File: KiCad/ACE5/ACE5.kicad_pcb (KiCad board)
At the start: 2 copper layers, 160 x 100 mm, 90 parts, among them Q1 2N3904, Q3 BC237, U1 LM7805_TO220, X1 CRYSTALHC49U-V 6.556MHz, X2 5MHz

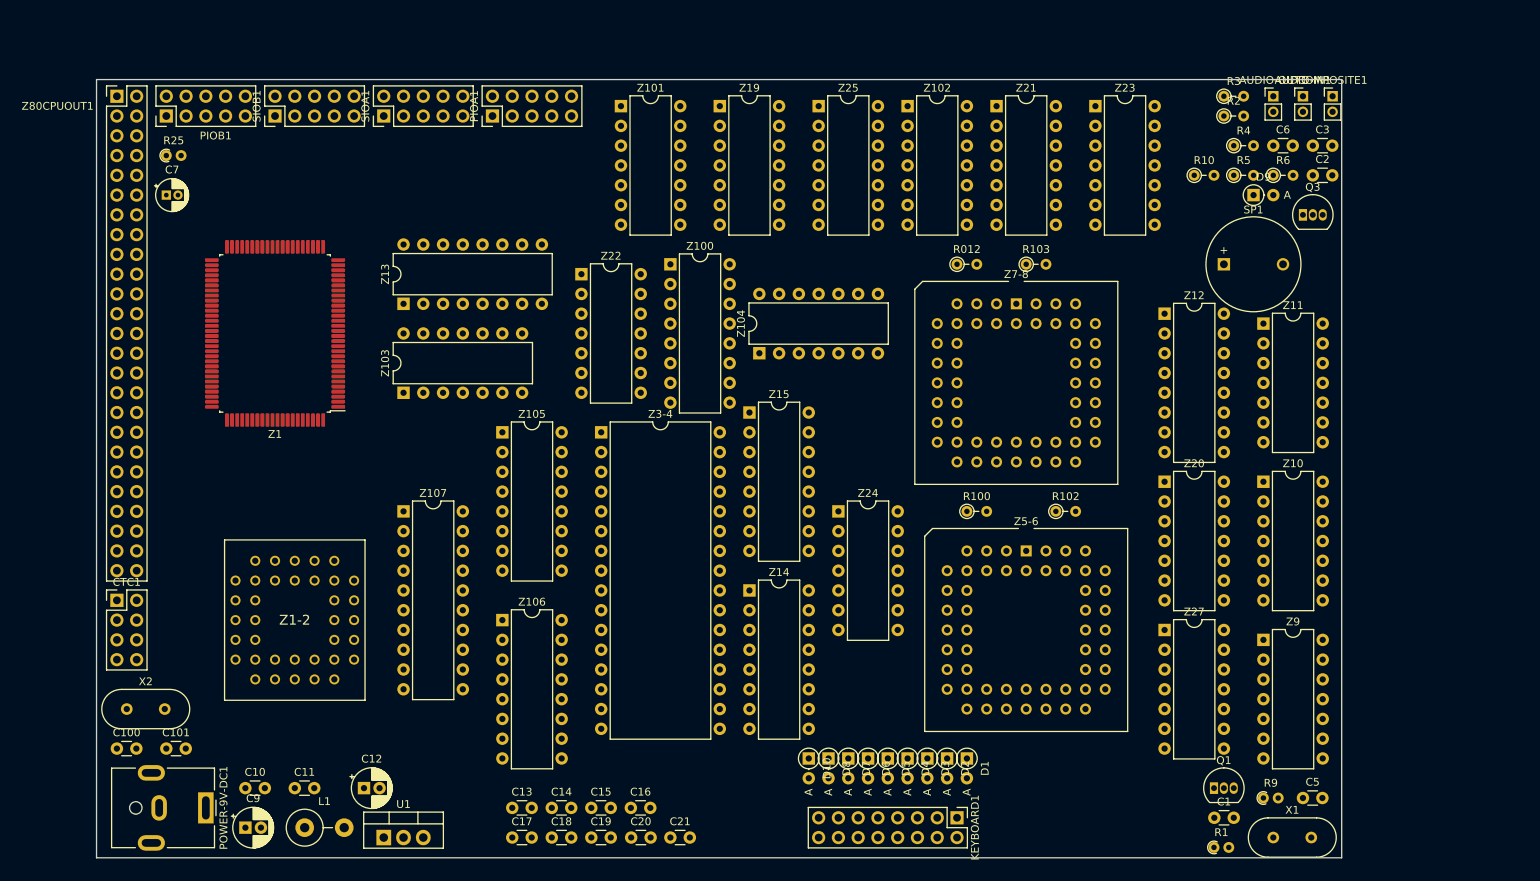
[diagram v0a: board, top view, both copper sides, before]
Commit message: UPdate to latest version.
Signed-off-by: John Bradley <flypie@rocketmail.com>
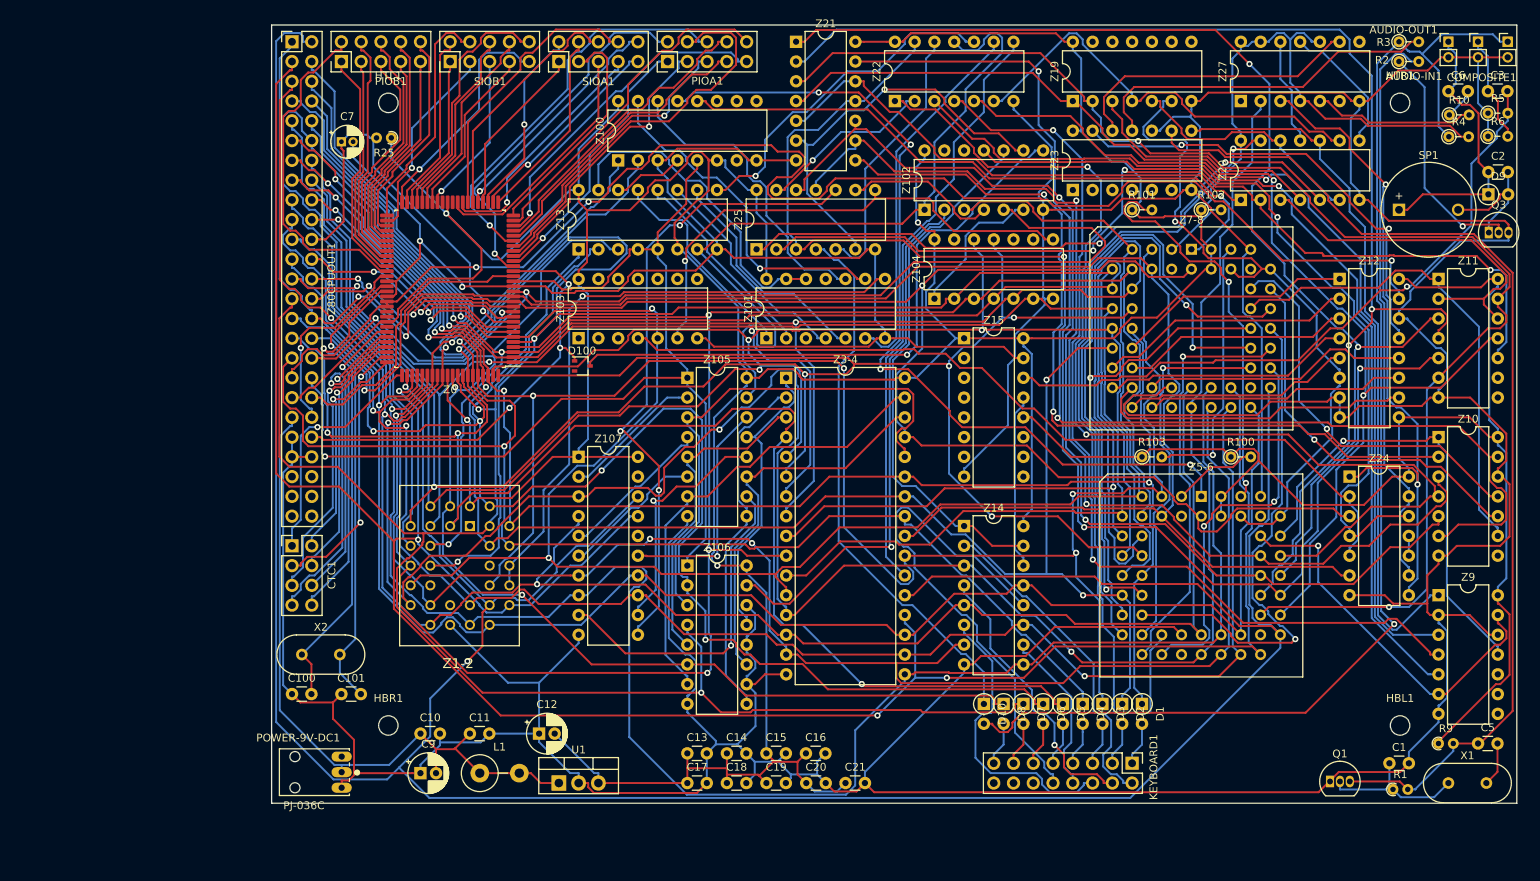
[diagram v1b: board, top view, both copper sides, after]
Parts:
- added D100: BAT54W, Package_TO_SOT_SMD:SOT-323_SC-70, F.Cu at (130.9, 91.8)
- added HBL1: MountingHole, MountingHole:MountingHole_2.5mm, F.Cu at (236.0, 138.0)
- added HBR1: MountingHole, MountingHole:MountingHole_2.5mm, F.Cu at (106.0, 138.0)
- added HTL1: MountingHole, MountingHole:MountingHole_2.5mm, F.Cu at (106.0, 58.0)
- added HTR1: MountingHole, MountingHole:MountingHole_2.5mm, F.Cu at (236.0, 58.0)
- L1: value L -> 100 nH
- POWER-9V-DC1: value Conn_01x02 -> PJ-036C; footprint Connector_BarrelJack:BarrelJack_CUI_PJ-063AH_Horizontal -> cuipj:CUI_PJ-036C
- moved Z27 68.7 mm to (215.5, 57.8), turned to 90 degrees
- moved Z24 65.8 mm to (229.5, 106.0)
- moved Z22 46.0 mm to (171.1, 57.8), turned to 90 degrees
- moved Z19 45.4 mm to (193.9, 57.8), turned to 90 degrees
- moved R101 40.0 mm to (201.6, 71.7)
- moved Z20 37.5 mm to (215.5, 70.5), turned to 90 degrees
- moved Z101 35.2 mm to (154.6, 88.2), turned to 90 degrees
- moved R100 34.6 mm to (214.3, 103.5)
- moved R10 33.7 mm to (242.3, 59.5)
- moved R5 33.6 mm to (247.3, 59.3)
- moved R102 32.2 mm to (210.5, 71.7)
- moved D9 30.2 mm to (247.3, 69.8)
- moved Z15 29.2 mm to (180.0, 88.2)
- moved R25 29.0 mm to (106.4, 62.5), turned to 180 degrees
- moved R103 28.9 mm to (202.8, 103.5)
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- renumbered R102 to R101, R012 to R102, Z1 to Z0
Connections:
- Z1-2 pad 16: Net-(Z1-2-Pad16) -> GND
- Z102 pad 8: //INT -> Net-(D100-Pad3)
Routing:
- net GND: track 0.00 -> 947.6 mm, vias 0 -> 2
- net +5V: track 0.00 -> 789.6 mm, vias 0 -> 4
- net /DA7: track 0.00 -> 410.8 mm, vias 0 -> 2
- net /DA0: track 0.00 -> 323.2 mm, vias 0 -> 4
- net /DA6: track 0.00 -> 309.5 mm, vias 0 -> 4
- net /A1: track 0.00 -> 293.2 mm, vias 0 -> 2
- net /A4: track 0.00 -> 280.4 mm, vias 0 -> 2
- net /A2: track 0.00 -> 279.4 mm, vias 0 -> 3
- net /A6: track 0.00 -> 267.9 mm, vias 0 -> 5
- net /A0: track 0.00 -> 266.7 mm, vias 0 -> 3
- net /A7: track 0.00 -> 261.7 mm, vias 0 -> 3
- net /A10: track 0.00 -> 252.7 mm, vias 0 -> 6
- net /DA2: track 0.00 -> 250.5 mm, vias 0 -> 4
- net //WR: track 0.00 -> 250.4 mm, vias 0 -> 3
- net /DA3: track 0.00 -> 244.1 mm, vias 0 -> 1
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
